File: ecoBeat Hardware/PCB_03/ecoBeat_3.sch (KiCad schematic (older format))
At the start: 24 parts, among them IC1 ATTINY85-P, J1 RJ45, P1 CONN_01X06, P3 CONN_01X02, SW1 SW_PUSH, SW2 SW_PUSH, U1 ESP-12E, U2 AP1117D33

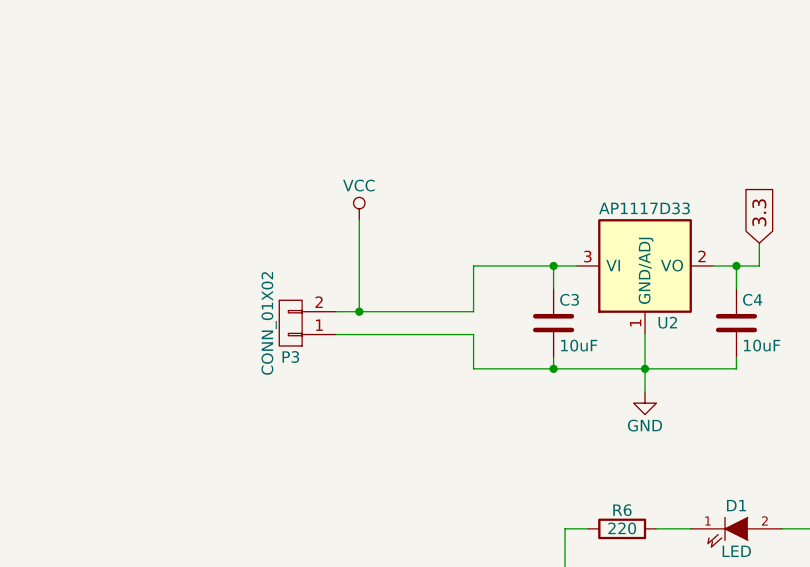
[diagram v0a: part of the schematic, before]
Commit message: gerber
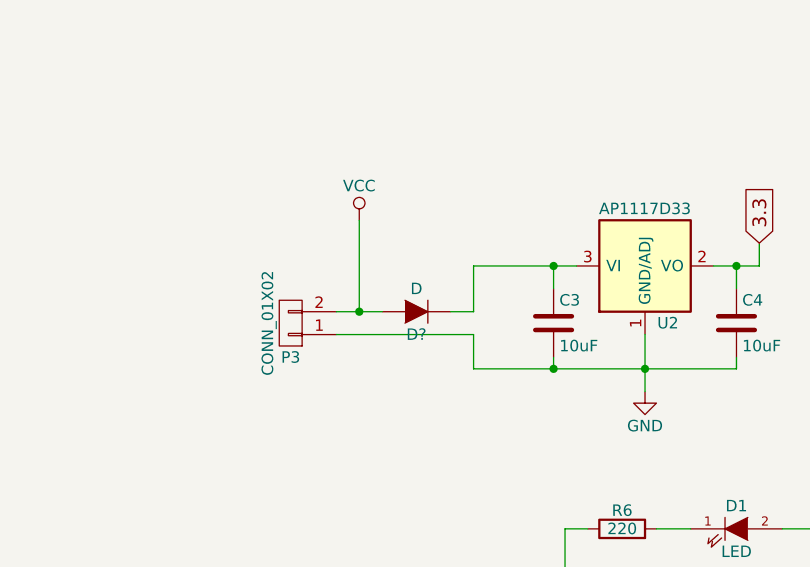
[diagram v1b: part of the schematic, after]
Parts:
- added D?: D, symbol D
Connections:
- net VCC: now also D?.2 (A); no longer C3.1, U2.3 (VI)
- new net: C3.1, D?.1 (K), U2.3 (VI)
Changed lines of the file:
@@
 	8200 3950 8200 3750
 Wire Wire Line
-	7600 3950 8200 3950
+	7600 3950 7800 3950
 Wire Wire Line
 	7600 4050 8200 4050
@@
 $EndComp
 Wire Wire Line
-	7700 3550 7700 3950
+	7700 3950 7700 3550
 Connection ~ 7700 3950
 Wire Wire Line
 	4700 2250 5150 2250
+$Comp
+L D D?
+U 1 1 5AAA6483
+P 7950 3950
+F 0 "D?" H 7950 4050 50  0000 C CNN
+F 1 "D" H 7950 3850 50  0000 C CNN
+F 2 "" H 7950 3950 50  0000 C CNN
+F 3 "" H 7950 3950 50  0000 C CNN
+	1    7950 3950
+	-1   0    0    1
+$EndComp
+Wire Wire Line
+	8200 3950 8100 3950
 $EndSCHEMATC
